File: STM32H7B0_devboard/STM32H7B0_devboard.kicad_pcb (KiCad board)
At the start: 4 copper layers, 60.4 x 90.4 mm, 101 parts, among them J1 SWD, J2 24LC512 socet, J3 USB-C 16P, Q1 S8050, Q2 AO3401A, SW1 BOOT_SEL, U1 STM32H7B0VBT6, U5 USBLC6-2SC6, Y1 32.768KHz, Y2 25MHz

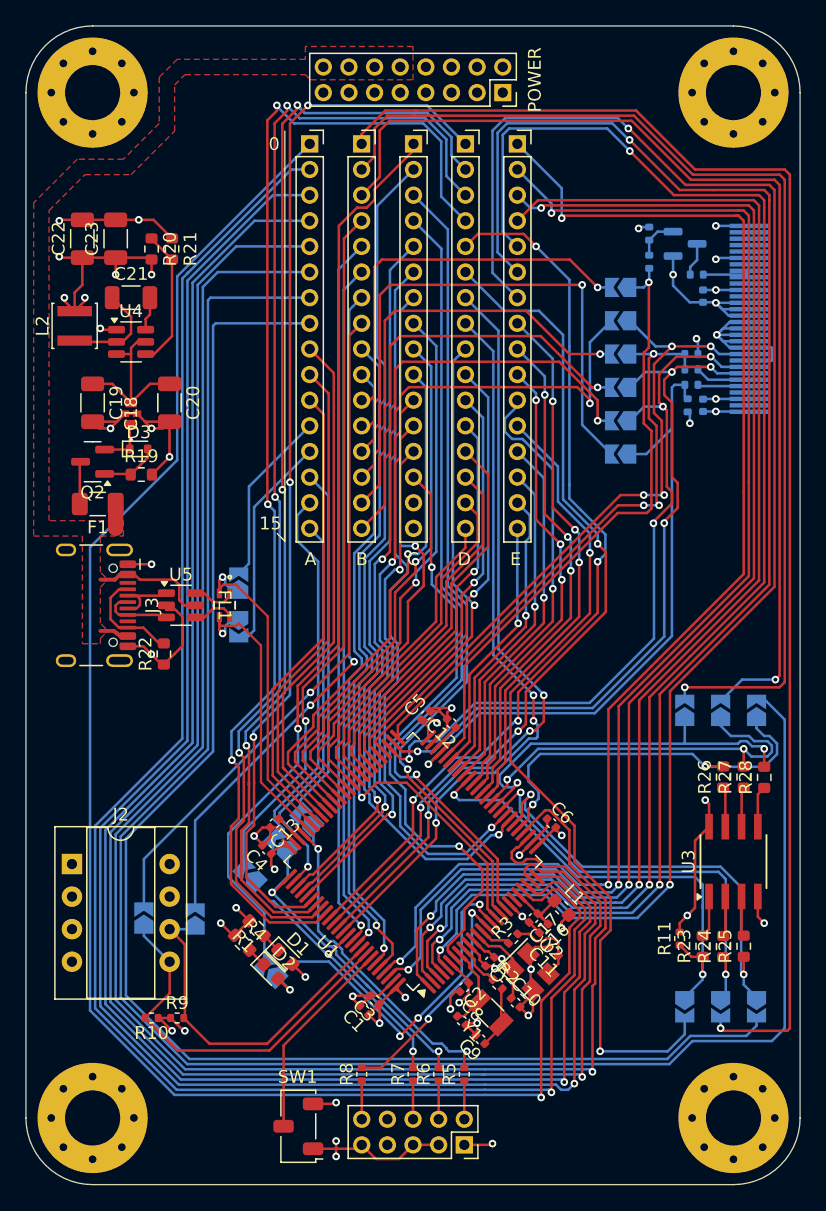
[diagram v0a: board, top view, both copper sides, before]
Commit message: Silk screen progress
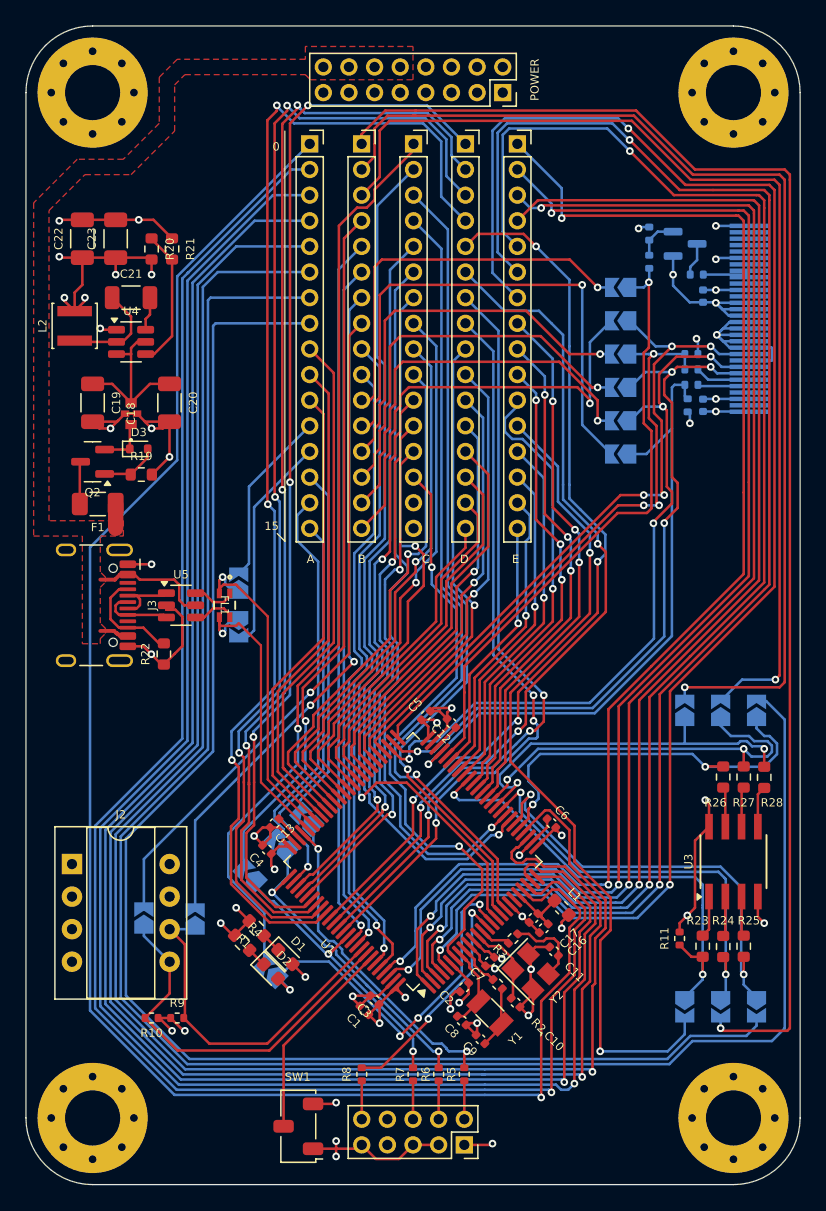
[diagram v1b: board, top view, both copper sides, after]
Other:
- board text added: ","
